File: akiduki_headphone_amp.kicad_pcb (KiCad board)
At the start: 2 copper layers, 62.8 x 41.8 mm, 22 parts, among them J1 IN, J2 OUT, U1 NJM4558

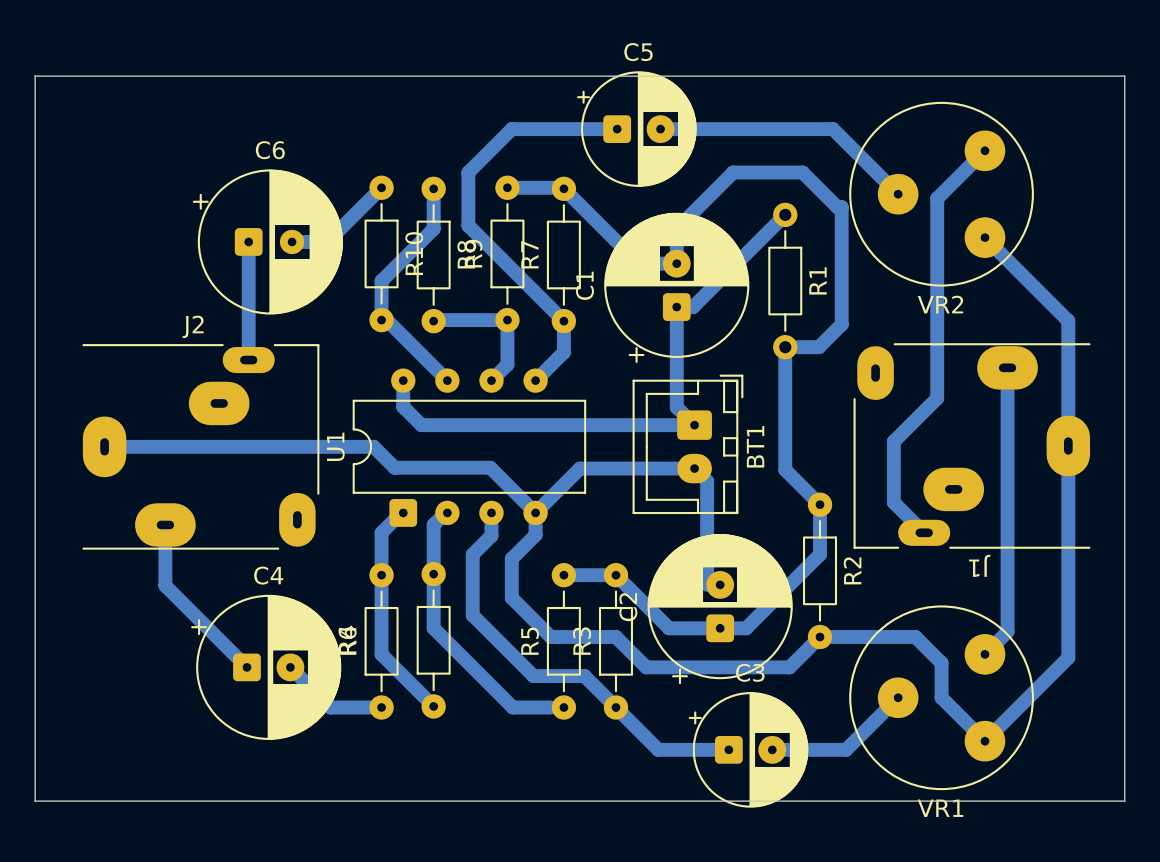
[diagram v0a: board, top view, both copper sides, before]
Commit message: パーツ間を詰めた
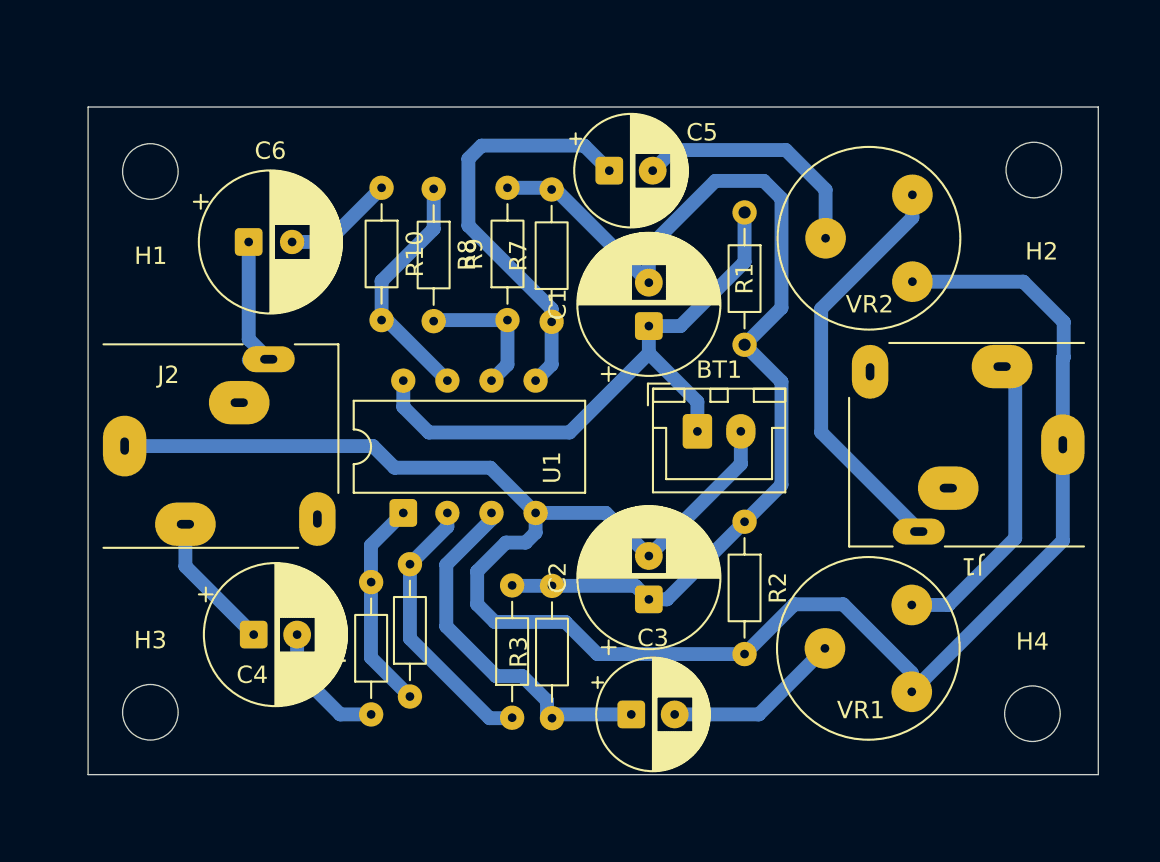
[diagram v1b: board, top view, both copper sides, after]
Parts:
- added H1: MountingHole, MountingHole:MountingHole_3.2mm_M3, F.Cu at (121.1, 81.0)
- added H2: MountingHole, MountingHole:MountingHole_3.2mm_M3, F.Cu at (172.0, 80.9)
- added H3: MountingHole, MountingHole:MountingHole_3.2mm_M3, F.Cu at (121.1, 112.1)
- added H4: MountingHole, MountingHole:MountingHole_3.2mm_M3, F.Cu at (171.9, 112.2)
- moved C3 5.98 mm to (148.8, 112.3)
- moved VR1 5.09 mm to (165.0, 106.0)
- moved VR2 4.89 mm to (165.0, 82.3)
- moved R2 4.46 mm to (155.4, 101.2)
- moved C2 4.43 mm to (149.8, 105.6)
- moved R3 3.74 mm to (144.3, 112.5)
- moved R5 3.04 mm to (142.0, 112.4)
- moved C5 2.44 mm to (147.6, 80.9)
- moved R1 2.35 mm to (155.4, 83.4)
- moved C1 1.94 mm to (149.8, 89.9)
- moved C4 1.93 mm to (127.1, 107.7)
- moved R4 1.48 mm to (136.1, 111.2)
- moved J2 1.15 mm to (119.7, 96.8)
- moved R6 0.72 mm to (133.8, 112.3)
- moved R7 0.71 mm to (144.2, 89.6)
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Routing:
- net VCC: track 66.3 -> 59.3 mm
- net Net-(U1A-+): track 24.3 -> 21.0 mm
- net Net-(C4-Pad1): track 10.1 -> 7.99 mm
- net Net-(C3-Pad2): track 8.49 -> 10.2 mm
- net Net-(C4-Pad2): track 6.21 -> 7.44 mm
- net GND: track 115.3 -> 114.2 mm
- net Net-(C5-Pad2): track 15.2 -> 14.2 mm
- net Net-(J1-PadR): track 24.9 -> 23.9 mm
- net +9V: track 34.4 -> 35.3 mm
- net Net-(R4-Pad1): track 13.0 -> 12.3 mm
- net Net-(J1-PadT): track 17.0 -> 17.7 mm
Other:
- board size 62.8 x 41.8 mm -> 58.2 x 38.4 mm
